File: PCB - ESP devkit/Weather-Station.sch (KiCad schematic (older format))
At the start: 28 parts, among them J1 Biruta, J10 Conn_01x19, J11 Conn_01x19, J2 Power, J3 BH1750-FVI, J4 BME280, J5 Pluviometro, J6 Anemometro, J8 Conn_01x02, J9 Conn_01x02, U1 AP1117-33

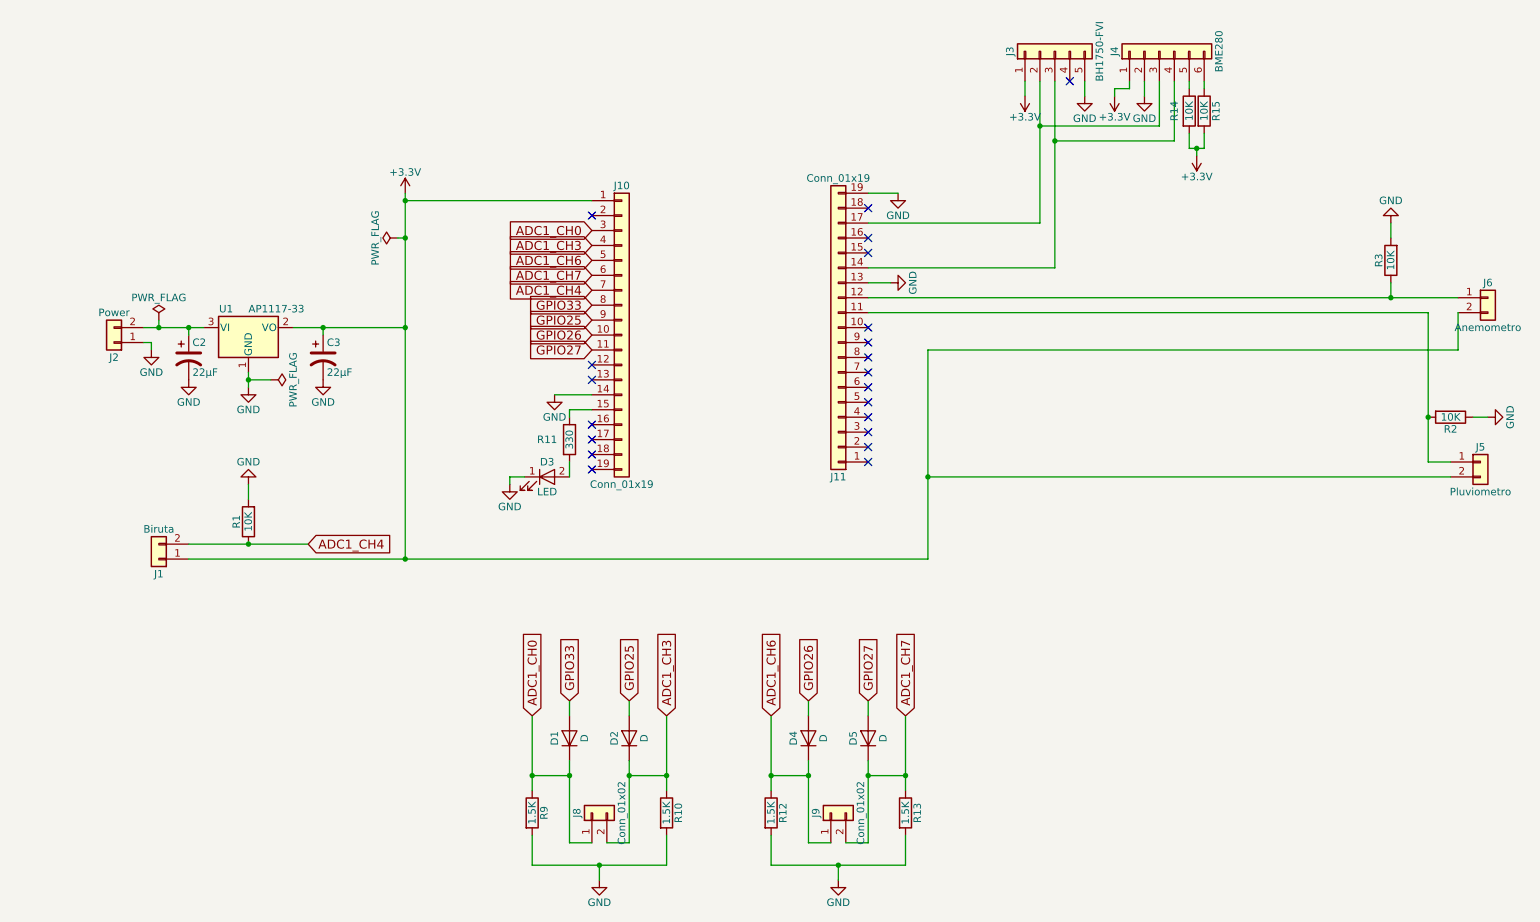
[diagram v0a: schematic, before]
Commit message: Ajustando PCBs
Signed-off-by: Gustavo Costa <gustavocosta@ic.ufal.br>
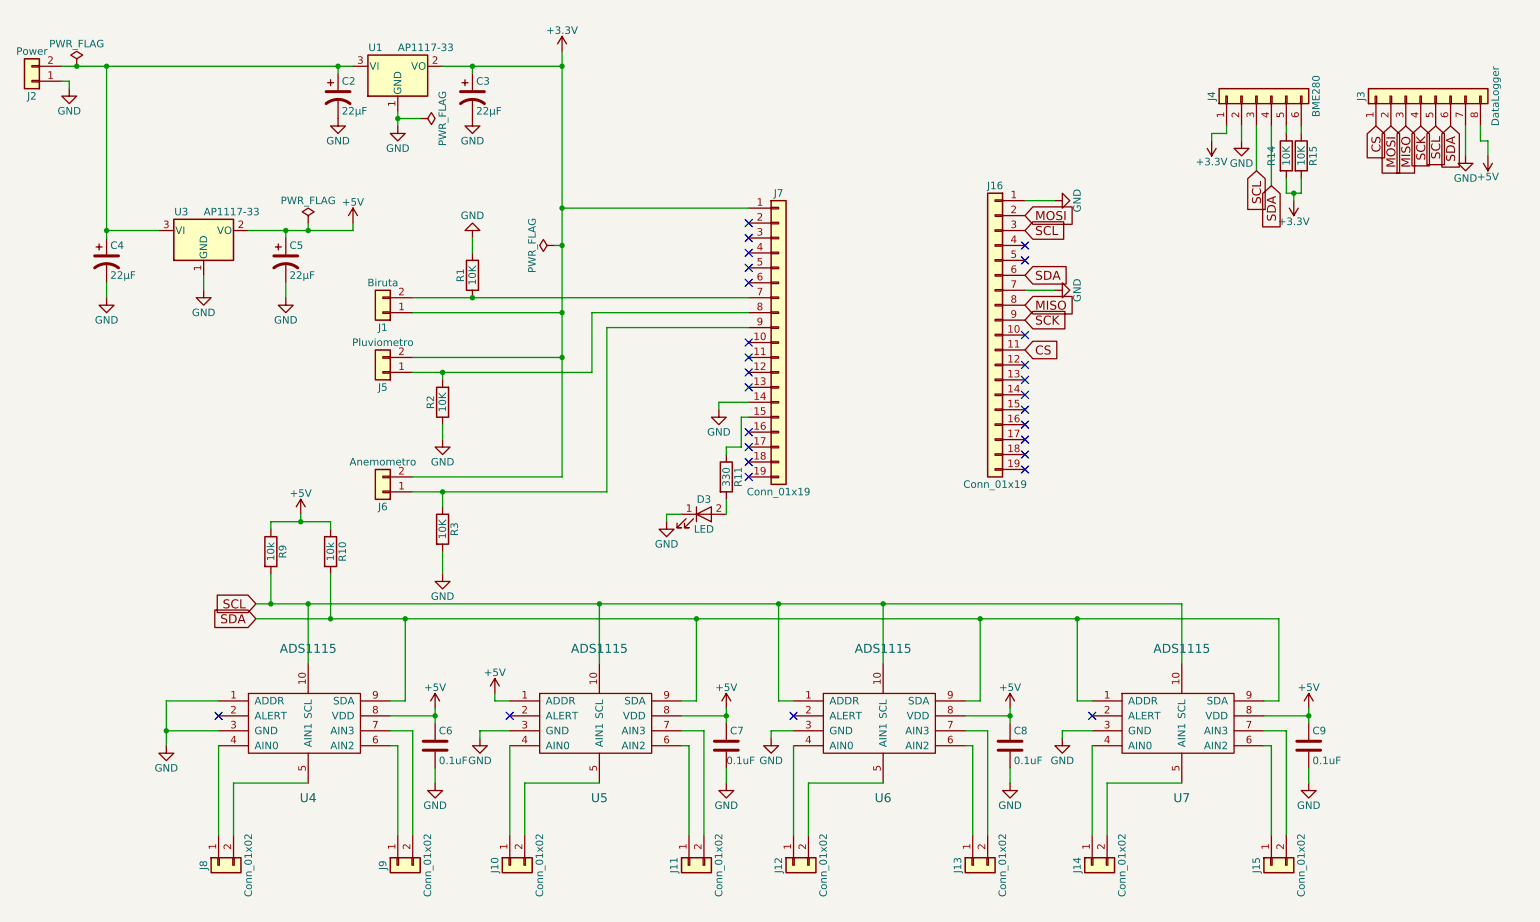
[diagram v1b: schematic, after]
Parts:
- removed D1, D2, D4, D5: D, Diodes_SMD:D_SOD-123, symbol D
- removed J10, J11: Conn_01x19, Pin_Headers:Pin_Header_Straight_1x19_Pitch2.54mm, symbol Conn_01x19
- removed J3: BH1750-FVI, TerminalBlock_Phoenix:TerminalBlock_Phoenix_MPT-2.54mm_5pol, symbol Conn_01x05
- removed R12, R13: 1.5K, Resistors_SMD:R_0805, symbol R
- added C4, C5: 22μF, Capacitors_SMD:CP_Elec_6.3x7.7, symbol CP1
- added C6, C7, C8, C9: 0.1uF, Capacitors_SMD:C_0805, symbol C
- added J10, J11, J12, J13, J14, J15: Conn_01x02, TerminalBlock_Phoenix:TerminalBlock_Phoenix_MPT-2.54mm_2pol, symbol Conn_01x02
- added J16, J7: Conn_01x19, Pin_Headers:Pin_Header_Straight_1x19_Pitch2.54mm, symbol Conn_01x19
- added J3: DataLogger, Pin_Headers:Pin_Header_Straight_1x08_Pitch2.54mm, symbol Conn_01x08
- added U3: AP1117-33, TO_SOT_Packages_SMD:SOT-223, symbol AP1117-33
- added U4, U5, U6, U7: ADS1115, Housings_SSOP:MSOP-10_3x3mm_Pitch0.5mm, symbol ADS1115
- J2: footprint TerminalBlock_Phoenix:TerminalBlock_Phoenix_MPT-2.54mm_2pol -> TerminalBlock_Phoenix:TerminalBlock_Phoenix_PT-3.5mm_2pol
- R10, R9: value 1.5K -> 10k
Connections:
- net +3V3: now also J7.1 (Pin_1)
- net GND: now also C4.2, C5.2, C6.2, C7.2, C8.2, C9.2, J16.1 (Pin_1), J16.7 (Pin_7), J3.7 (Pin_7), J7.14 (Pin_14), U3.1 (GND), U4.1 (ADDR), U4.3 (GND), U5.3 (GND), U6.3 (GND), U7.3 (GND); no longer R10.2, R9.2
- net at J6.1 (Pin_1), R3.1: now also J7.9 (Pin_9)
- net at J5.1 (Pin_1), R2.2: now also J7.8 (Pin_8)
- net SCL: now reaches J4.3 (Pin_3)
- net SCL: now also R9.2, J16.3 (Pin_3), J3.5 (Pin_5), U4.10 (SCL), U5.10 (SCL), U6.1 (ADDR), U6.10 (SCL), U7.10 (SCL)
- net SDA: now reaches J4.4 (Pin_4)
- net SDA: now also R10.2, J16.6 (Pin_6), J3.6 (Pin_6), U4.9 (SDA), U5.9 (SDA), U6.9 (SDA), U7.1 (ADDR), U7.9 (SDA)
- net at C2.1, J2.2 (Pin_2), U1.3 (VI): now also C4.1, U3.3 (VI)
- net at R11.1: now also J7.15 (Pin_15)
- net ADC1_CH0: no longer names the net of J8.1 (Pin_1)
- net ADC1_CH0: now also U4.4 (AIN0); no longer R9.1
- net ADC1_CH3: no longer names the net of J8.2 (Pin_2)
- net ADC1_CH3: now also U4.5 (AIN1); no longer R10.1
- net ADC1_CH4: no longer names the net of J1.2 (Pin_2), R1.1
- net ADC1_CH4: now also J7.7 (Pin_7)
- net ADC1_CH6: no longer names the net of J9.1 (Pin_1)
- net ADC1_CH6: now also U4.6 (AIN2)
- net ADC1_CH7: no longer names the net of J9.2 (Pin_2)
- net ADC1_CH7: now also U4.7 (AIN3)
- new net: J10.1 (Pin_1), U5.4 (AIN0)
- new net: J10.2 (Pin_2), U5.5 (AIN1)
- new net: J11.1 (Pin_1), U5.6 (AIN2)
- new net: J11.2 (Pin_2), U5.7 (AIN3)
- new net: J12.1 (Pin_1), U6.4 (AIN0)
- new net: J12.2 (Pin_2), U6.5 (AIN1)
- new net: J13.1 (Pin_1), U6.6 (AIN2)
- new net: J13.2 (Pin_2), U6.7 (AIN3)
- new net: J14.1 (Pin_1), U7.4 (AIN0)
- new net: J14.2 (Pin_2), U7.5 (AIN1)
- new net: J15.1 (Pin_1), U7.6 (AIN2)
- new net: J15.2 (Pin_2), U7.7 (AIN3)
- new net +5V: C5.1, C6.1, C7.1, C8.1, C9.1, J3.8 (Pin_8), R10.1, R9.1, U3.2 (VO), U4.8 (VDD), U5.1 (ADDR), U5.8 (VDD), U6.8 (VDD), U7.8 (VDD)
- new net CS: J16.11 (Pin_11), J3.1 (Pin_1)
- new net MISO: J16.8 (Pin_8), J3.3 (Pin_3)
- new net MOSI: J16.2 (Pin_2), J3.2 (Pin_2)
- new net SCK: J16.9 (Pin_9), J3.4 (Pin_4)
- no-connect marks 21 -> 28
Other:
- moved on the sheet: C2, C3, D3, J1, J2, J4, J5, J6, R1, R11, R14, R15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
